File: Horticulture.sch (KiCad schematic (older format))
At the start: 66 parts, among them J2 Conn_02x05_Odd_Even, J3 Conn_01x04_Male, J4 Conn_01x04_Male, SW1 SW-I2C, SW2 Rotary_Encoder_Switch, U1 TLE4309, U2 TLE4309, U3 TLE4309, U4 TLE4309, U6 STM32F030F4Px, U7 SSD1306

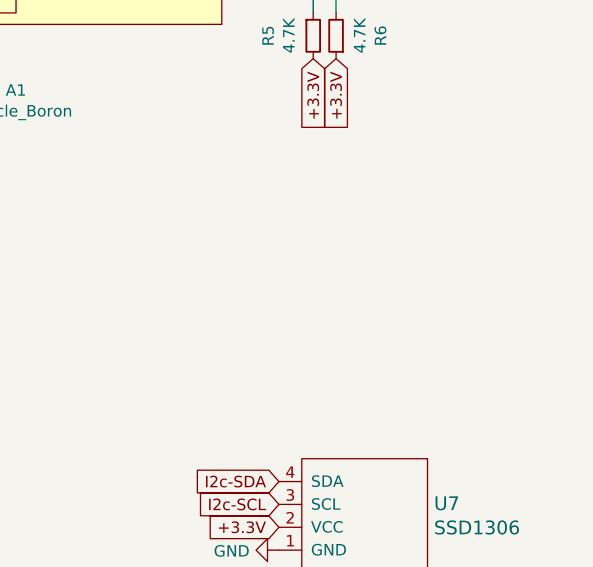
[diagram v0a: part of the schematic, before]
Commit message: 3.2.1- RC2. Fixes #4
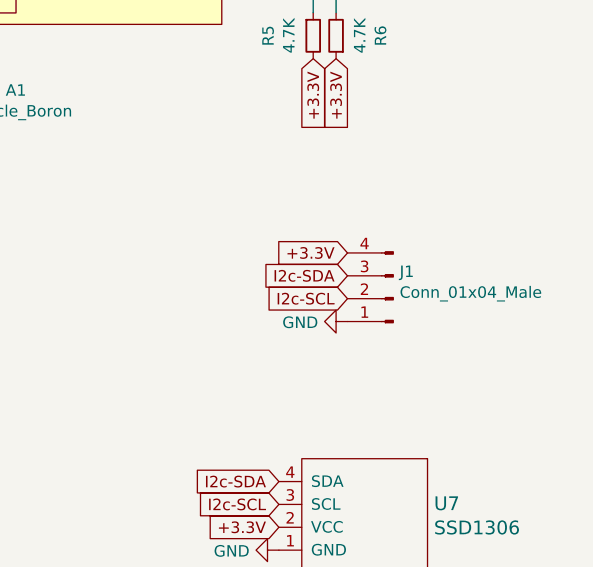
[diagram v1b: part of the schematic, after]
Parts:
- added J1: Conn_01x04_Male, Connector_Molex:Molex_PicoBlade_53398-0471_1x04-1MP_P1.25mm_Vertical, symbol Connector:Conn_01x04_Male
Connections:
- net +3.3V: now also J1.4 (Pin_4)
- net GND: now also J1.1 (Pin_1)
- net I2c-SCL: now also J1.2 (Pin_2)
- net I2c-SDA: now also J1.3 (Pin_3)
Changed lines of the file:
@@
 Wire Wire Line
 	8200 6950 8150 6950
+Text GLabel 13650 5300 0    50   Input ~ 0
++3.3V
+$Comp
+L power:GND #PWR0126
+U 1 1 5FCD9F7E
+P 13650 5600
+F 0 "#PWR0126" H 13650 5350 50  0001 C CNN
+F 1 "GND" V 13655 5472 50  0000 R CNN
+F 2 "" H 13650 5600 50  0001 C CNN
+F 3 "" H 13650 5600 50  0001 C CNN
+	1    13650 5600
+	0    1    1    0
+$EndComp
+Text GLabel 13650 5500 0    50   Input ~ 0
+I2c-SCL
+Text GLabel 13650 5400 0    50   Input ~ 0
+I2c-SDA
+$Comp
+L Connector:Conn_01x04_Male J1
+U 1 1 5FCECF34
+P 13850 5500
+F 0 "J1" H 13822 5382 50  0000 R CNN
+F 1 "Conn_01x04_Male" H 13822 5473 50  0000 R CNN
+F 2 "Connector_Molex:Molex_PicoBlade_53398-0471_1x04-1MP_P1.25mm_Vertical" H 13850 5500 50  0001 C CNN
+F 3 "~" H 13850 5500 50  0001 C CNN
+	1    13850 5500
+	-1   0    0    1
+$EndComp
 $EndSCHEMATC
